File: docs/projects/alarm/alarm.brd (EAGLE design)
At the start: 39 x 41.9 mm, 8 parts, among them IC2 MEGA8-P

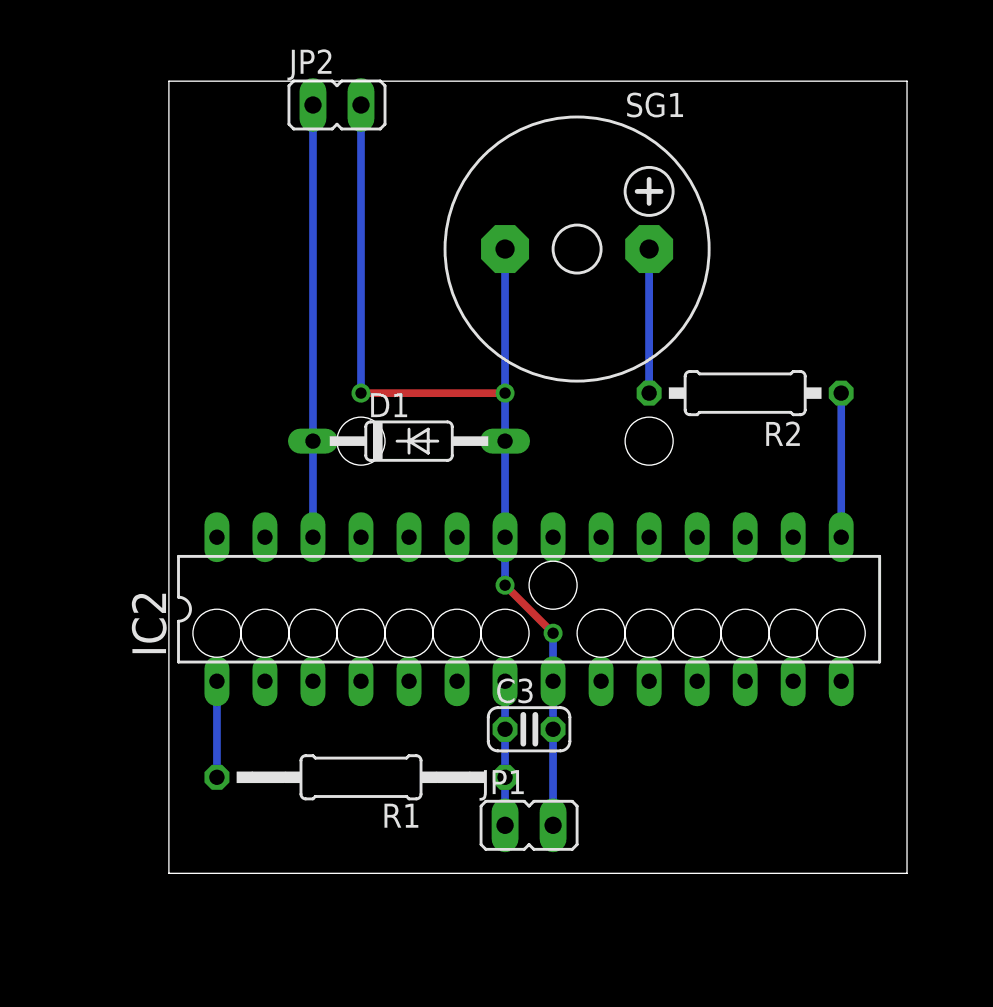
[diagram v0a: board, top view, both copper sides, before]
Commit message: alarm: new debug
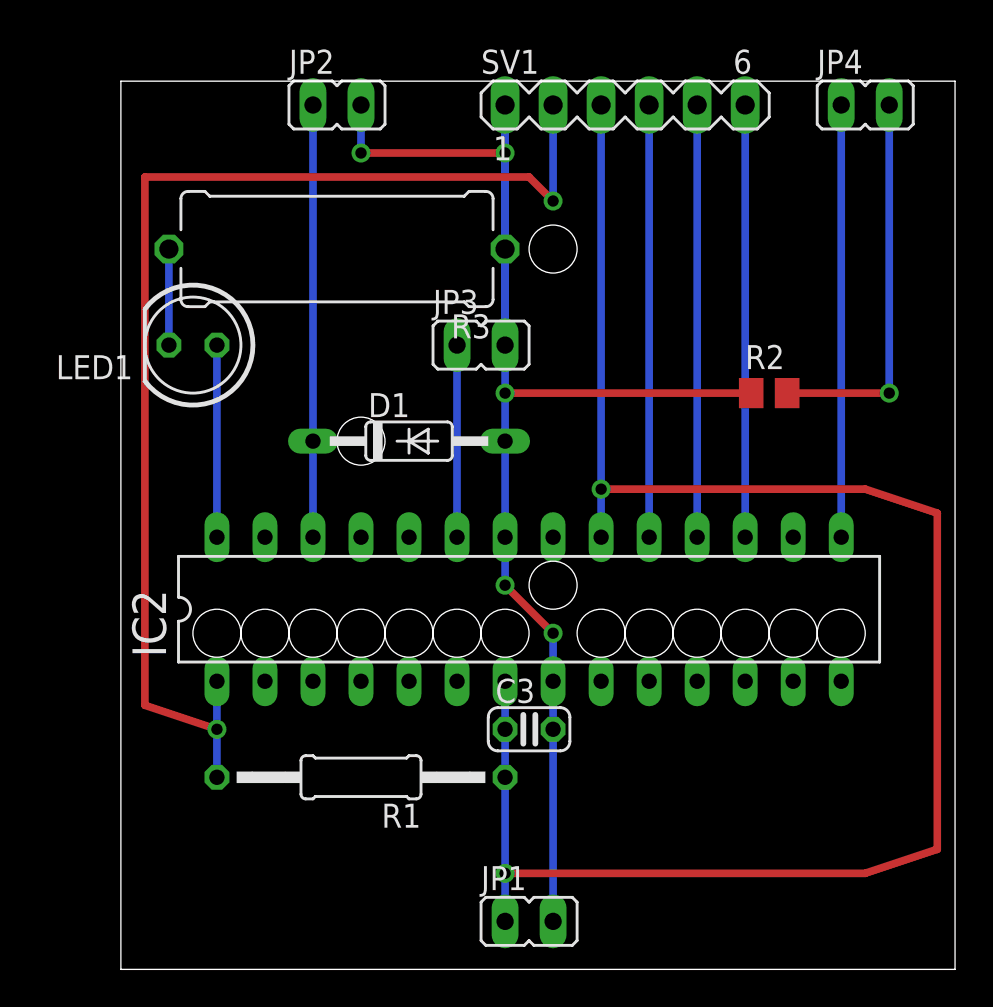
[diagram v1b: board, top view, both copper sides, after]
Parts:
- removed SG1: F/CM12P, buzzer:F/CM12P
- added JP3: DEBUG, jumper:JP1
- added JP4: SPEAKER, jumper:JP1
- added LED1: DEBUG, led:LED5MM
- added R3: 1k, rcl:0617/17
- added SV1: (no value), con-lstb:MA06-1
- R2: device rcl:0207/10 -> rcl:M0805
- moved JP1 5.08 mm to (36.8, 0.00)
- moved R2 1.27 mm to (49.5, 27.9), turned to 0 degrees
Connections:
- removed net AVCC: IC2.20
- new net N$4: IC2.23, JP3.1
- new net N$5: IC2.19, SV1.4
- new net N$6: IC2.18, SV1.5
- new net N$7: IC2.17, SV1.6
- new net N$8: LED1.K, R3.2
- new net N$9: IC2.28, LED1.A
- net GND: now also JP3.2, R2.1, R3.1, SV1.1; no longer SG1.-
- net N$1: now also JP4.2; no longer SG1.+
- net N$17: now also SV1.2
- net N$3: now also JP4.1; no longer R2.1
- net VCC: now also IC2.20, SV1.3
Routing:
- net VCC: track 7.62 -> 94.4 mm, vias 0 -> 2
- net N$17: track 5.08 -> 64.2 mm, vias 0 -> 2
- net GND: track 54.4 -> 87.7 mm, vias 4 -> 5
- net N$7: track 0.00 -> 22.9 mm
- net N$6: track 0.00 -> 22.9 mm
- net N$5: track 0.00 -> 22.9 mm
- net N$3: track 7.62 -> 22.9 mm
- net N$1: track 7.62 -> 20.6 mm, vias 0 -> 1
- net N$9: track 0.00 -> 10.2 mm
- net N$4: track 0.00 -> 10.2 mm
- net N$8: track 0.00 -> 5.08 mm
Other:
- board size 39 x 41.9 mm -> 44.1 x 47 mm
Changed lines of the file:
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@@
 <board>
 <plain>
-<wire x1="17.78" y1="2.54" x2="56.82" y2="2.54" width="0" layer="20"/>
-<wire x1="56.82" y1="2.54" x2="56.82" y2="44.44" width="0" layer="20"/>
-<wire x1="56.82" y1="44.44" x2="17.78" y2="44.44" width="0" layer="20"/>
-<wire x1="17.78" y1="44.44" x2="17.78" y2="2.54" width="0" layer="20"/>
+<wire x1="15.24" y1="-2.54" x2="59.36" y2="-2.54" width="0" layer="20"/>
+<wire x1="59.36" y1="-2.54" x2="59.36" y2="44.44" width="0" layer="20"/>
+<wire x1="59.36" y1="44.44" x2="15.24" y2="44.44" width="0" layer="20"/>
+<wire x1="15.24" y1="44.44" x2="15.24" y2="-2.54" width="0" layer="20"/>
 <hole x="53.34" y="15.24" drill="2.54"/>
 <hole x="50.8" y="15.24" drill="2.54"/>
@@
 <hole x="20.32" y="15.24" drill="2.54"/>
 <hole x="35.56" y="15.24" drill="2.54"/>
-<hole x="43.18" y="25.4" drill="2.54"/>
+<hole x="38.1" y="35.56" drill="2.54"/>
 <hole x="27.94" y="25.4" drill="2.54"/>
 </plain>
@@
 <element name="R1" library="rcl" package="0207/15" value="10k" x="27.94" y="7.62" rot="R180"/>
 <element name="D1" library="diode" package="DO35-10" value="1N4148DO35-10" x="30.48" y="25.4"/>
-<element name="SG1" library="buzzer" package="F/CM12P" value="F/CM12P" x="39.37" y="35.56">
-<attribute name="MF" value="" x="39.37" y="35.56" size="1.778" layer="27" display="off"/>
-<attribute name="MPN" value="" x="39.37" y="35.56" size="1.778" layer="27" display="off"/>
-<attribute name="OC_FARNELL" value="unknown" x="39.37" y="35.56" size="1.778" layer="27" display="off"/>
-<attribute name="OC_NEWARK" value="unknown" x="39.37" y="35.56" size="1.778" layer="27" display="off"/>
+<element name="R2" library="rcl" package="M0805" value="100" x="49.53" y="27.94"/>
+<element name="JP1" library="jumper" package="JP1" value="POWER" x="36.83" y="0" rot="R270"/>
+<element name="JP2" library="jumper" package="JP1" value="IN" x="26.67" y="43.18" rot="R270"/>
+<element name="JP3" library="jumper" package="JP1" value="DEBUG" x="34.29" y="30.48" rot="R270"/>
+<element name="SV1" library="con-lstb" package="MA06-1" value="" x="41.91" y="43.18">
+<attribute name="OC_NEWARK" value="unknown" x="41.91" y="43.18" size="1.778" layer="27" display="off"/>
+<attribute name="MPN" value="" x="41.91" y="43.18" size="1.778" layer="27" display="off"/>
+<attribute name="MF" value="" x="41.91" y="43.18" size="1.778" layer="27" display="off"/>
+<attribute name="OC_FARNELL" value="unknown" x="41.91" y="43.18" size="1.778" layer="27" display="off"/>
 </element>
-<element name="R2" library="rcl" package="0207/10" value="100" x="48.26" y="27.94" rot="R180"/>
-<element name="JP1" library="jumper" package="JP1" value="POWER" x="36.83" y="5.08" rot="R270"/>
-<element name="JP2" library="jumper" package="JP1" value="IN" x="26.67" y="43.18" rot="R270"/>
+<element name="LED1" library="led" package="LED5MM" value="DEBUG" x="19.05" y="30.48" rot="R180"/>
+<element name="R3" library="rcl" package="0617/17" value="1k" x="26.67" y="35.56" rot="R180"/>
+<element name="JP4" library="jumper" package="JP1" value="SPEAKER" x="54.61" y="43.18" rot="R270"/>
 </elements>
 <signals>
@@
 <contactref element="IC2" pad="22"/>
 <contactref element="C3" pad="2"/>
-<contactref element="SG1" pad="-"/>
 <contactref element="D1" pad="A"/>
 <contactref element="JP1" pad="2"/>
@@
 <wire x1="35.56" y1="20.32" x2="35.56" y2="25.4" width="0.4064" layer="16"/>
 <wire x1="35.56" y1="25.4" x2="35.56" y2="27.94" width="0.4064" layer="16"/>
-<wire x1="35.56" y1="27.94" x2="35.56" y2="35.56" width="0.4064" layer="16"/>
+<wire x1="35.56" y1="27.94" x2="35.56" y2="40.64" width="0.4064" layer="16"/>
 <wire x1="38.1" y1="10.16" x2="38.1" y2="12.7" width="0.4064" layer="16"/>
-<wire x1="38.1" y1="5.08" x2="38.1" y2="10.16" width="0.4064" layer="16"/>
-<wire x1="27.94" y1="27.94" x2="27.94" y2="43.18" width="0.4064" layer="16"/>
-<wire x1="35.56" y1="27.94" x2="27.94" y2="27.94" width="0.4064" layer="1"/>
+<wire x1="38.1" y1="0" x2="38.1" y2="10.16" width="0.4064" layer="16"/>
+<wire x1="27.94" y1="40.64" x2="27.94" y2="43.18" width="0.4064" layer="16"/>
+<wire x1="35.56" y1="40.64" x2="27.94" y2="40.64" width="0.4064" layer="1"/>
 <via x="35.56" y="17.78" extent="1-16" drill="0.6" shape="square"/>
 <via x="38.1" y="15.24" extent="1-16" drill="0.6" shape="square"/>
-<via x="27.94" y="27.94" extent="1-16" drill="0.6" shape="square"/>
+<via x="27.94" y="40.64" extent="1-16" drill="0.6" shape="square"/>
+<via x="35.56" y="40.64" extent="1-16" drill="0.6" shape="square"/>
+<contactref element="JP3" pad="2"/>
+<contactref element="SV1" pad="1"/>
+<wire x1="35.56" y1="40.64" x2="35.56" y2="43.18" width="0.4064" layer="16"/>
+<wire x1="35.56" y1="43.18" x2="35.56" y2="30.48" width="0.4064" layer="16"/>
+<contactref element="R3" pad="1"/>
+<wire x1="35.56" y1="43.18" x2="35.56" y2="35.56" width="0.4064" layer="16"/>
+<contactref element="R2" pad="1"/>
 <via x="35.56" y="27.94" extent="1-16" drill="0.6" shape="square"/>
+<wire x1="48.58" y1="27.94" x2="35.56" y2="27.94" width="0.4064" layer="1"/>
 </signal>
 <signal name="VCC">
@@
 <wire x1="35.56" y1="10.16" x2="35.56" y2="12.7" width="0.4064" layer="16"/>
 <wire x1="35.56" y1="7.62" x2="35.56" y2="10.16" width="0.4064" layer="16"/>
-<wire x1="35.56" y1="5.08" x2="35.56" y2="7.62" width="0.4064" layer="16"/>
+<wire x1="35.56" y1="0" x2="35.56" y2="2.54" width="0.4064" layer="16"/>
+<contactref element="SV1" pad="3"/>
+<contactref element="IC2" pad="20"/>
+<wire x1="35.56" y1="2.54" x2="35.56" y2="7.62" width="0.4064" layer="16"/>
+<wire x1="40.64" y1="43.18" x2="40.64" y2="22.86" width="0.4064" layer="16"/>
+<wire x1="40.64" y1="22.86" x2="40.64" y2="20.32" width="0.4064" layer="16"/>
+<via x="40.64" y="22.86" extent="1-16" drill="0.6" shape="square"/>
+<via x="35.56" y="2.54" extent="1-16" drill="0.6" shape="square"/>
+<wire x1="35.56" y1="2.54" x2="54.61" y2="2.54" width="0.4064" layer="1"/>
+<wire x1="54.61" y1="2.54" x2="58.42" y2="3.81" width="0.4064" layer="1"/>
+<wire x1="58.42" y1="3.81" x2="58.42" y2="21.59" width="0.4064" layer="1"/>
+<wire x1="58.42" y1="21.59" x2="54.61" y2="22.86" width="0.4064" layer="1"/>
+<wire x1="54.61" y1="22.86" x2="40.64" y2="22.86" width="0.4064" layer="1"/>
 </signal>
 <signal name="N$17">
 <contactref element="IC2" pad="1"/>
 <contactref element="R1" pad="2"/>
-<wire x1="20.32" y1="7.62" x2="20.32" y2="12.7" width="0.4064" layer="16"/>
-</signal>
-<signal name="AVCC">
-<contactref element="IC2" pad="20"/>
-</signal>
-<signal name="N$1">
-<contactref element="R2" pad="2"/>
-<contactref element="SG1" pad="+"/>
-<wire x1="43.18" y1="27.94" x2="43.18" y2="35.56" width="0.4064" layer="16"/>
+<wire x1="20.32" y1="7.62" x2="20.32" y2="10.16" width="0.4064" layer="16"/>
+<contactref element="SV1" pad="2"/>
+<wire x1="20.32" y1="10.16" x2="20.32" y2="12.7" width="0.4064" layer="16"/>
+<wire x1="38.1" y1="43.18" x2="38.1" y2="38.1" width="0.4064" layer="16"/>
+<via x="38.1" y="38.1" extent="1-16" drill="0.6" shape="square"/>
+<via x="20.32" y="10.16" extent="1-16" drill="0.6" shape="square"/>
+<wire x1="38.1" y1="38.1" x2="36.83" y2="39.37" width="0.4064" layer="1"/>
+<wire x1="36.83" y1="39.37" x2="16.51" y2="39.37" width="0.4064" layer="1"/>
+<wire x1="16.51" y1="39.37" x2="16.51" y2="11.43" width="0.4064" layer="1"/>
+<wire x1="16.51" y1="11.43" x2="20.32" y2="10.16" width="0.4064" layer="1"/>
 </signal>
 <signal name="N$2">
@@
 <wire x1="25.4" y1="25.4" x2="25.4" y2="43.18" width="0.4064" layer="16"/>
 </signal>
+<signal name="N$5">
+<contactref element="IC2" pad="19"/>
+<contactref element="SV1" pad="4"/>
+<wire x1="43.18" y1="20.32" x2="43.18" y2="43.18" width="0.4064" layer="16"/>
+</signal>
+<signal name="N$6">
+<contactref element="IC2" pad="18"/>
+<contactref element="SV1" pad="5"/>
+<wire x1="45.72" y1="20.32" x2="45.72" y2="43.18" width="0.4064" layer="16"/>
+</signal>
+<signal name="N$7">
+<contactref element="IC2" pad="17"/>
+<contactref element="SV1" pad="6"/>
+<wire x1="48.26" y1="20.32" x2="48.26" y2="43.18" width="0.4064" layer="16"/>
+</signal>
+<signal name="N$4">
+<contactref element="JP3" pad="1"/>
+<contactref element="IC2" pad="23"/>
+<wire x1="33.02" y1="20.32" x2="33.02" y2="30.48" width="0.4064" layer="16"/>
+</signal>
+<signal name="N$8">
+<contactref element="LED1" pad="K"/>
+<contactref element="R3" pad="2"/>
+<wire x1="17.78" y1="30.48" x2="17.78" y2="35.56" width="0.4064" layer="16"/>
+</signal>
+<signal name="N$9">
+<contactref element="LED1" pad="A"/>
+<contactref element="IC2" pad="28"/>
+<wire x1="20.32" y1="30.48" x2="20.32" y2="20.32" width="0.4064" layer="16"/>
+</signal>
+<signal name="N$1">
+<contactref element="JP4" pad="2"/>
+<contactref element="R2" pad="2"/>
+<wire x1="55.88" y1="43.18" x2="55.88" y2="27.94" width="0.4064" layer="16"/>
+<via x="55.88" y="27.94" extent="1-16" drill="0.6" shape="square"/>
+<wire x1="50.48" y1="27.94" x2="55.88" y2="27.94" width="0.4064" layer="1"/>
+</signal>
 <signal name="N$3">
+<contactref element="JP4" pad="1"/>
 <contactref element="IC2" pad="15"/>
-<contactref element="R2" pad="1"/>
-<wire x1="53.34" y1="20.32" x2="53.34" y2="27.94" width="0.4064" layer="16"/>
+<wire x1="53.34" y1="20.32" x2="53.34" y2="43.18" width="0.4064" layer="16"/>
 </signal>
 </signals>
